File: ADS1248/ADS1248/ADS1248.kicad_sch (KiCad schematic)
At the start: 23 parts

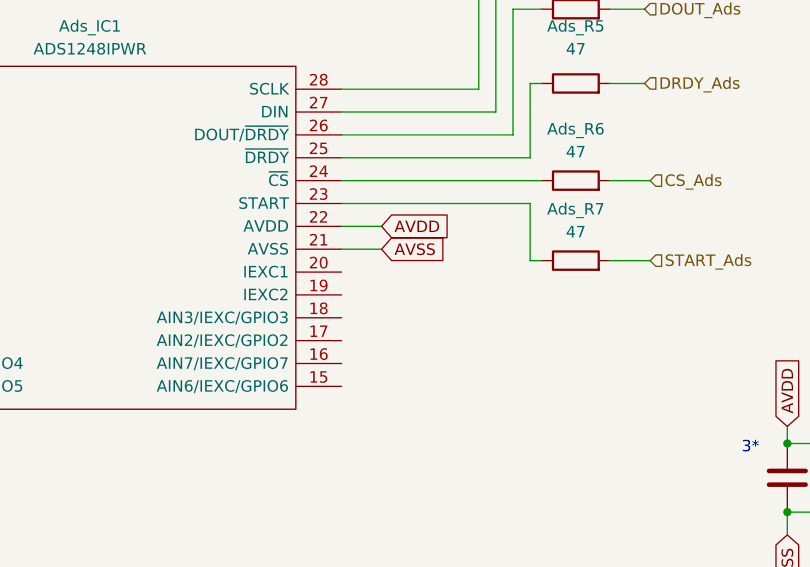
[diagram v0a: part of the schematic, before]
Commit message: updates ads1115 and ads 1248
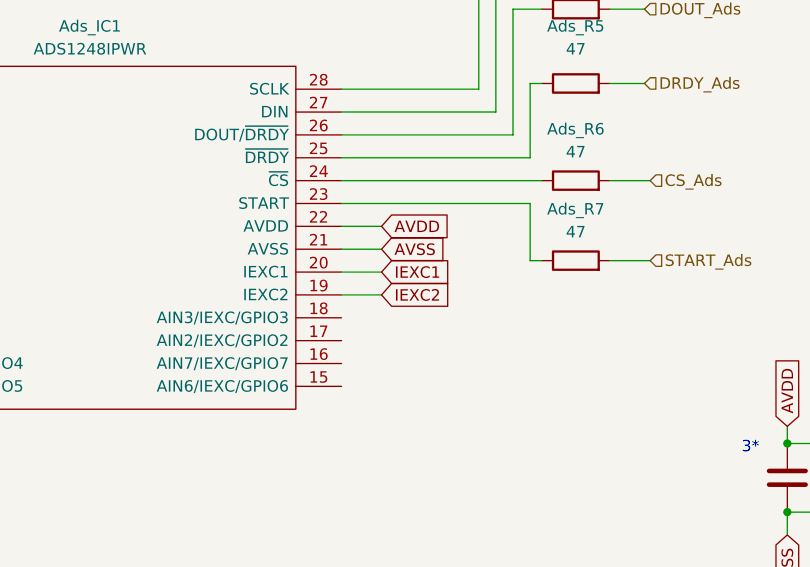
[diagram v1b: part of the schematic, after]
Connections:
- net AIN2: now also Ads_IC1.20 (IEXC1)
- net AIN3: now also Ads_IC1.19 (IEXC2)
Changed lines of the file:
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@@
+    (stroke (width 0) (type default))
+  )
+  (wire (pts (xy 313.055 85.725) (xy 308.61 85.725))
     (stroke (width 0) (type default))
   )
@@
   )
   (wire (pts (xy 338.455 73.025) (xy 342.9 73.025))
+    (stroke (width 0) (type default))
+  )
+  (wire (pts (xy 313.055 83.185) (xy 308.61 83.185))
     (stroke (width 0) (type default))
   )
@@
     )
   )
+  (global_label "IEXC2" (shape input) (at 313.055 85.725 0) (fields_autoplaced)
+    (effects (font (size 1.27 1.27)) (justify left))
+    (property "Intersheetrefs" "${INTERSHEET_REFS}" (at 321.483 85.725 0)
+      (effects (font (size 1.27 1.27)) (justify left) hide)
+    )
+  )
   (global_label "VRefOut" (shape input) (at 203.2 90.17 90) (fields_autoplaced)
     (effects (font (size 1.27 1.27)) (justify left))
@@
       (effects (font (size 1.27 1.27)) (justify left) hide)
     )
+  )
+  (global_label "IEXC1" (shape input) (at 313.055 83.185 0) (fields_autoplaced)
+    (effects (font (size 1.27 1.27)) (justify left))
+    (property "Intersheetrefs" "${INTERSHEET_REFS}" (at 321.483 83.185 0)
+      (effects (font (size 1.27 1.27)) (justify left) hide)
+    )

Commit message: add ads1248, RTD multiple sensors 2 wires
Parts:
- removed CRTD_I_CM1, CRTD_I_CM2, CRTD_I_DIFF, CR_CM1, CR_CM2, CR_CM_DIFF: C, symbol Device:C
- removed REF, RR1, RR2, RRTD_I1, RRTD_I2, RTD: R, symbol Device:R
- added Ads_ain_C1, Ads_ain_C2, Ads_ain_C3, Ads_ain_C4, Ads_ain_C5, Ads_ain_C6, Ads_ref_0_C1, Ads_ref_0_C2, Ads_ref_0_C3, Ads_ref_1_C1, Ads_ref_1_C2: 0.1uF, Capacitor_SMD:C_0603_1608Metric, symbol Device:C
- added CRTD_I_CM5, CRTD_I_CM6, CRTD_I_DIFF3: C, Capacitor_SMD:C_0603_1608Metric, symbol Device:C
- added JP_+1, JP_-1, JP_IEXC1, JP_ain0, JP_gnd1, JP_ref_5, JP_ref_refp1: Jumper_2_Open, Jumper:SolderJumper-2_P1.3mm_Open_TrianglePad1.0x1.5mm, symbol Jumper:Jumper_2_Open
- added REF1: 10K, Resistor_SMD:R_0603_1608Metric, symbol Device:R
- added Ref_C1, Ref_C3: 1uF, Capacitor_SMD:C_0603_1608Metric, symbol Device:C
- added Ref_C2: 22uF, Capacitor_SMD:C_0603_1608Metric, symbol Device:C
- added U1: REF5050AD, Package_SO:SOIC-8_3.9x4.9mm_P1.27mm, symbol Reference_Voltage:REF5050AD
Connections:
- net GND: now also Ads_IC1.8 (REFN1), Ads_ain_C1.1, Ads_ain_C3.2, Ads_ain_C4.1, Ads_ain_C6.2, Ads_ref_0_C1.1, Ads_ref_0_C3.2, Ads_ref_1_C1.1, Ads_ref_1_C2.2, CRTD_I_CM5.1, CRTD_I_CM6.2, JP_gnd1.2 (B), Ref_C1.1, Ref_C2.2, Ref_C3.2, U1.4 (GND)
- net REFN0: now also Ads_IC1.6 (REFN0/GPIO1), Ads_ref_0_C2.2, Ads_ref_0_C3.1, REF1.1
- net REFP0: now also Ads_IC1.14 (AIN5/IEXC/GPIO5), Ads_IC1.17 (AIN2/IEXC/GPIO2), Ads_IC1.5 (REFP0/GPIO0), Ads_ain_C2.2, Ads_ain_C3.1, Ads_ain_C5.2, Ads_ain_C6.1, Ads_ref_0_C1.2, Ads_ref_0_C2.1, REF1.2
- net VRefOut: now also Ads_C2.1; no longer Ads_C3.1
- net ain0: now reaches Ads_IC1.11 (AIN0/IEXC)
- net ain0: now also JP_ain0.1 (A)
- net ain1: now reaches Ads_IC1.12 (AIN1/IEXC)
- net ain1: now also Ads_ain_C4.2, Ads_ain_C5.1, JP_IEXC1.2 (B), JP_ain0.2 (B)
- net ain3: now reaches Ads_IC1.13 (AIN4/IEXC/GPIO4)
- net ain3: now also Ads_IC1.18 (AIN3/IEXC/GPIO3), Ads_ain_C1.2, Ads_ain_C2.1
- net ain6: now reaches Ads_IC1.15 (AIN6/IEXC/GPIO6)
- net ain6: now also CRTD_I_CM5.2, CRTD_I_DIFF3.1, JP_+1.2 (B)
- net ain7: now reaches Ads_IC1.16 (AIN7/IEXC/GPIO7)
- net ain7: now also CRTD_I_CM6.1, CRTD_I_DIFF3.2, JP_-1.2 (B)
- net REFP1: now reaches Ads_IC1.7 (REFP1)
- net REFP1: now also Ads_ref_1_C1.2, Ads_ref_1_C2.1, JP_ref_refp1.2 (B)
- net +5V renamed +5V_ref
- net +5V_ref: now also Ads_C3.1, JP_ref_5.2 (B), JP_ref_refp1.1 (A), Ref_C2.1, U1.6 (Vout); no longer Ads_C2.1
- net AIN2 renamed IEXC1
- net IEXC1: now also JP_IEXC1.1 (A)
- net AIN3 renamed IEXC2
- new net: Ref_C3.1, U1.5 (Trim/NR)
- new net 5V: Ref_C1.2, U1.2 (Vin)
- new net sens_pressure_+: JP_+1.1 (A)
- new net sens_pressure_-: JP_-1.1 (A)
- new net sens_pressure_GND: JP_gnd1.1 (A)
- new net sens_pressure_ref_5V: JP_ref_5.1 (A)
- no-connect marks 0 -> 1
